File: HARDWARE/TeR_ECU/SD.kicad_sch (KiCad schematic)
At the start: 7 parts, among them J5 Micro_SD_Card

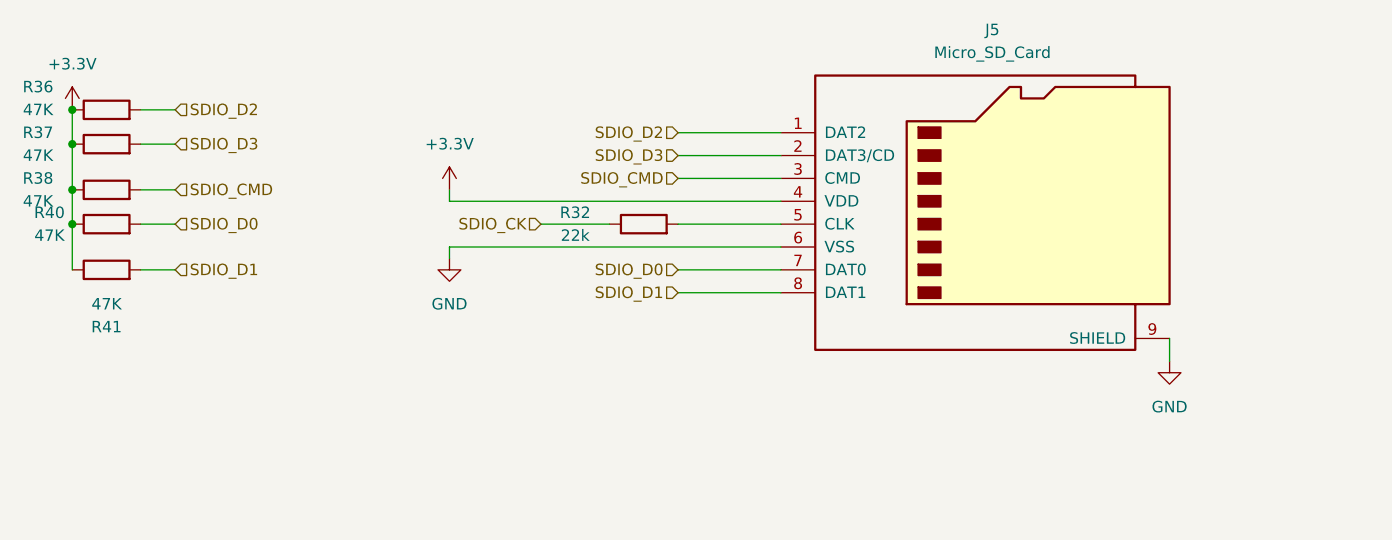
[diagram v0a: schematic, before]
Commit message: Kept improving schmatic for V2
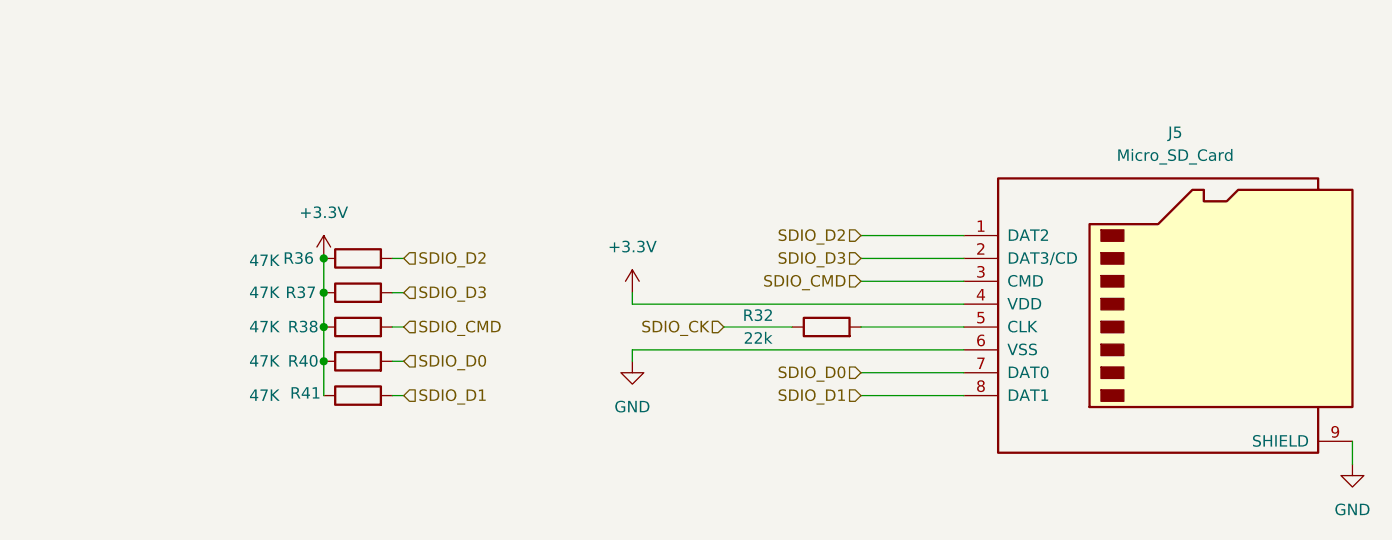
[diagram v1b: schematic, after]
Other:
- moved on the sheet: J5, R32, R36, R37, R38, R40, R41
